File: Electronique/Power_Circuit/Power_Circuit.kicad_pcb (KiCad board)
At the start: 2 copper layers, 40 parts, among them U1 B_Plug_5mm, U10 B_Plug_5mm, U11 B_Plug_5mm, U12 B_Plug_5mm, U13 B_Plug_5mm, U14 B_Plug_5mm, U15 DSN2596, U16 DSN2596, U17 B_Plug_5mm, U18 B_Plug_5mm, U2 B_Plug_5mm, U3 B_Plug_5mm, U4 trou-d3mm, U5 DSN2596, U6 trou-d3mm, U7 B_Plug_5mm, U8 trou-d3mm, U9 trou-d3mm

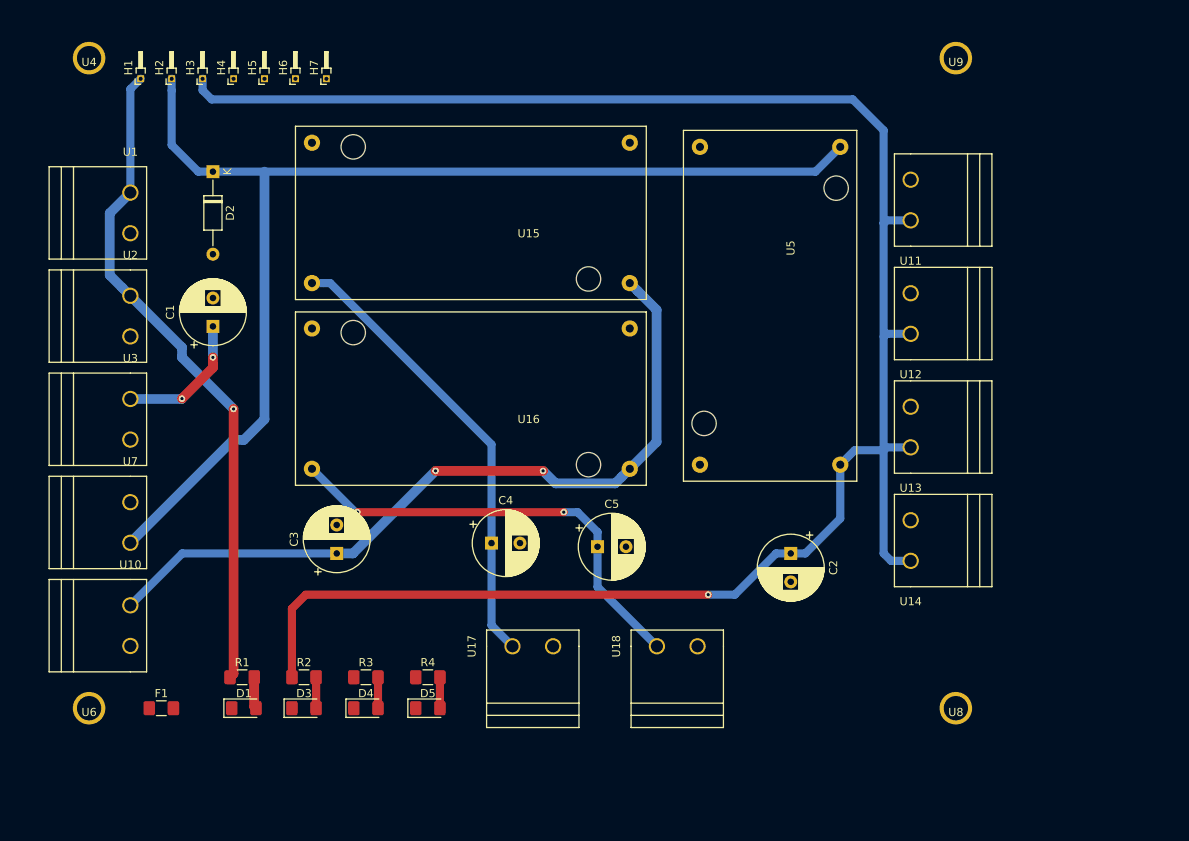
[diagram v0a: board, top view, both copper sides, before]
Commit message: Circuit adjustement
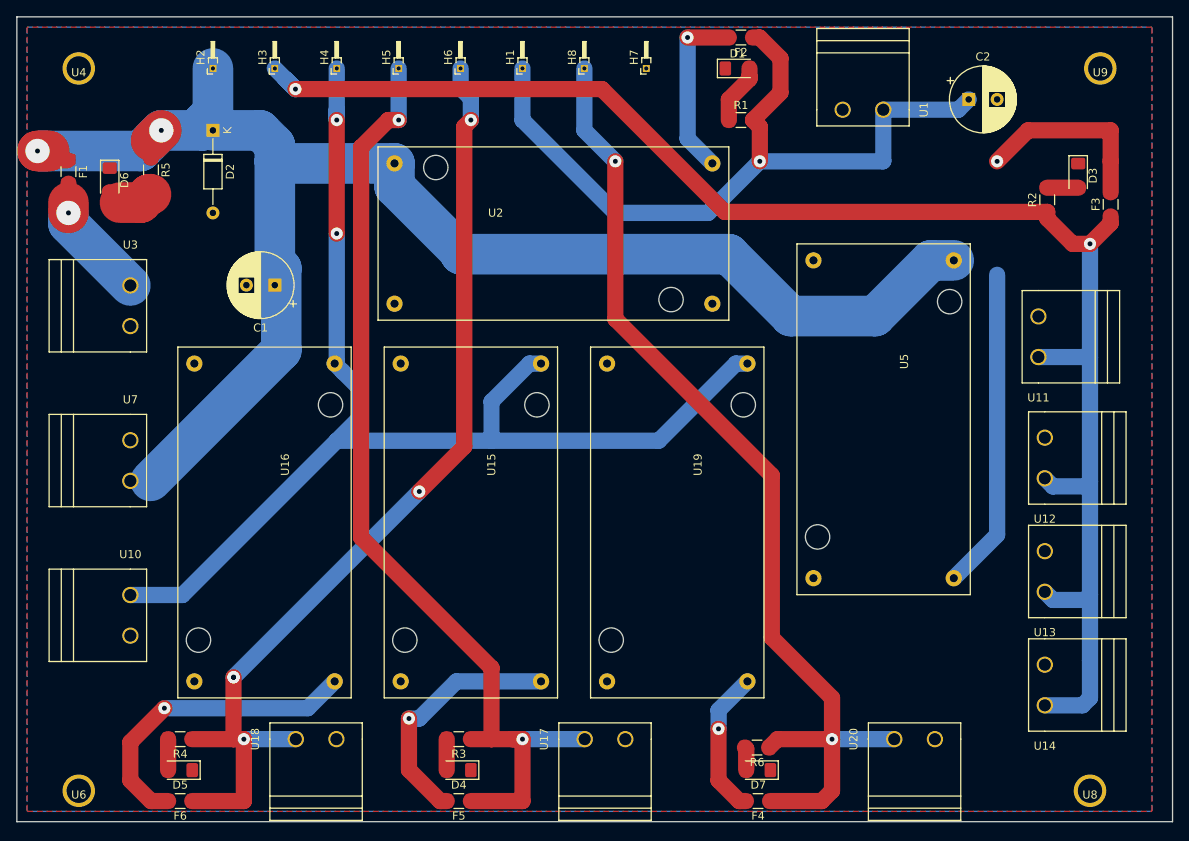
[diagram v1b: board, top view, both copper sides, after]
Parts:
- removed C3, C4, C5: CP, Capacitor_THT:CP_Radial_D8.0mm_P3.50mm
- added D6: LED, LED_SMD:LED_1206_3216Metric_Pad1.42x1.75mm_HandSolder, F.Cu at (24.1, 32.8)
- added D7: LED, LED_SMD:LED_1206_3216Metric_Pad1.42x1.75mm_HandSolder, F.Cu at (104.0, 105.4)
- added F2: Fuse, Fuse:Fuse_1206_3216Metric_Pad1.42x1.75mm_HandSolder, F.Cu at (101.8, 15.2)
- added F3: Fuse, Fuse:Fuse_1206_3216Metric_Pad1.42x1.75mm_HandSolder, F.Cu at (147.3, 35.8)
- added F4: Fuse, Fuse:Fuse_1206_3216Metric_Pad1.42x1.75mm_HandSolder, F.Cu at (103.9, 109.2)
- added F5: Fuse, Fuse:Fuse_1206_3216Metric_Pad1.42x1.75mm_HandSolder, F.Cu at (67.1, 109.2)
- added F6: Fuse, Fuse:Fuse_1206_3216Metric_Pad1.42x1.75mm_HandSolder, F.Cu at (32.8, 109.2)
- added H8: MountingHole_Pad, Connector_PinHeader_1.00mm:PinHeader_1x01_P1.00mm_Horizontal, F.Cu at (82.5, 19.1)
- added R5: R, Resistor_SMD:R_1206_3216Metric_Pad1.42x1.75mm_HandSolder, F.Cu at (29.2, 31.5)
- added R6: R, Resistor_SMD:R_1206_3216Metric_Pad1.42x1.75mm_HandSolder, F.Cu at (103.8, 102.6)
- added U19: DSN2596, dsn2596:DSN2596, F.Cu at (94.0, 74.9)
- added U20: B_Plug_5mm, dsn2596:B plug 5mm, F.Cu at (123.2, 101.6)
- U2: value B_Plug_5mm -> DSN2596; footprint dsn2596:B plug 5mm -> dsn2596:DSN2596
- moved D3 115.7 mm to (143.3, 32.2), turned to 270 degrees
- moved R2 108.7 mm to (139.5, 35.2), turned to 90 degrees
- moved D1 99.4 mm to (101.4, 19.1)
- moved R1 92.0 mm to (101.8, 25.4)
- moved U1 91.1 mm to (116.8, 24.1), turned to 270 degrees
- moved F1 67.0 mm to (19.1, 31.8), turned to 270 degrees
- moved C2 60.0 mm to (129.8, 22.9), turned to 0 degrees
- moved U2 53.1 mm to (78.7, 39.4)
- moved H1 47.0 mm to (74.9, 19.1)
- moved U18 45.9 mm to (49.5, 101.6)
- moved H7 39.4 mm to (90.2, 19.1)
- moved U15 38.1 mm to (68.6, 74.9), turned to 270 degrees
- moved D5 31.4 mm to (32.8, 105.4), turned to 180 degrees
- moved R4 31.4 mm to (32.8, 101.6), turned to 180 degrees
- moved U16 29.6 mm to (43.2, 74.9), turned to 270 degrees
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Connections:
- C1 pad 1: Net-(C1-Pad1) -> 18V
- C2 pad 1: Logical_10V -> Raspberr_5V
- F1 pad 2: Net-(C1-Pad1) -> Net-(F1-Pad2)
- H1 pad 1: Battery -> Raspberr_5V
- R1 pad 1: Battery -> Net-(D1-Pad2)
- R1 pad 2: Net-(D1-Pad2) -> Raspberr_5V
- U1 pad 1: Battery -> Raspberr_5V
- U15 pad 4: Motor1_12V -> Net-(F5-Pad2)
- U16 pad 4: Motor2_12V -> Net-(F6-Pad2)
- U2 pad 1: Battery -> 18V
- U3 pad 1: Net-(C1-Pad1) -> Net-(F1-Pad2)
- U5 pad 4: Logical_10V -> Net-(F3-Pad2)
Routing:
- net MotorExt_12V: track 0.00 -> 125.5 mm, vias 0 -> 2
- net Raspberr_5V: track 0.00 -> 94.3 mm, vias 0 -> 1
- net Battery: track 81.7 -> 0.00 mm, vias 1 -> 0
- net Motor2_12V: track 55.5 -> 121.9 mm, vias 2 -> 5
- net Motor1_12V: track 56.2 -> 122.4 mm, vias 0 -> 2
- net Net-(F3-Pad2): track 0.00 -> 62.7 mm, vias 0 -> 1
- net 12V: track 95.3 -> 151.4 mm
- net 18V: track 146.4 -> 200.1 mm, vias 0 -> 2
- net Logical_10V: track 246.7 -> 198.4 mm, vias 1 -> 2
- net Net-(F6-Pad2): track 0.00 -> 38.6 mm, vias 0 -> 1
- net Net-(F5-Pad2): track 0.00 -> 30.7 mm, vias 0 -> 1
- net Net-(F2-Pad2): track 0.00 -> 21.8 mm, vias 0 -> 1
- net Net-(F1-Pad2): track 0.00 -> 18.2 mm, vias 0 -> 1
- net Net-(F4-Pad2): track 0.00 -> 18.1 mm, vias 0 -> 1
- net Net-(C1-Pad1): track 16.8 -> 0.00 mm, vias 2 -> 0
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- added copper zone on B.Cu, net GND
- added copper zone on F.Cu, net GND
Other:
- board outline added: 142.2 x 99.1 mm
- net class Default: clearance 0.2 -> 1
- rule trace_clearance: 0.2 -> 1
